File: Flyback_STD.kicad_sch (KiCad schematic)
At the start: 46 parts, among them P1 BATT+, P2 BATT-, P3 VBUS, P4 GND, Q1 5N20A, T1 TRF-6, U1 OB2106MP, U2 VPC2188B, U4 TL431

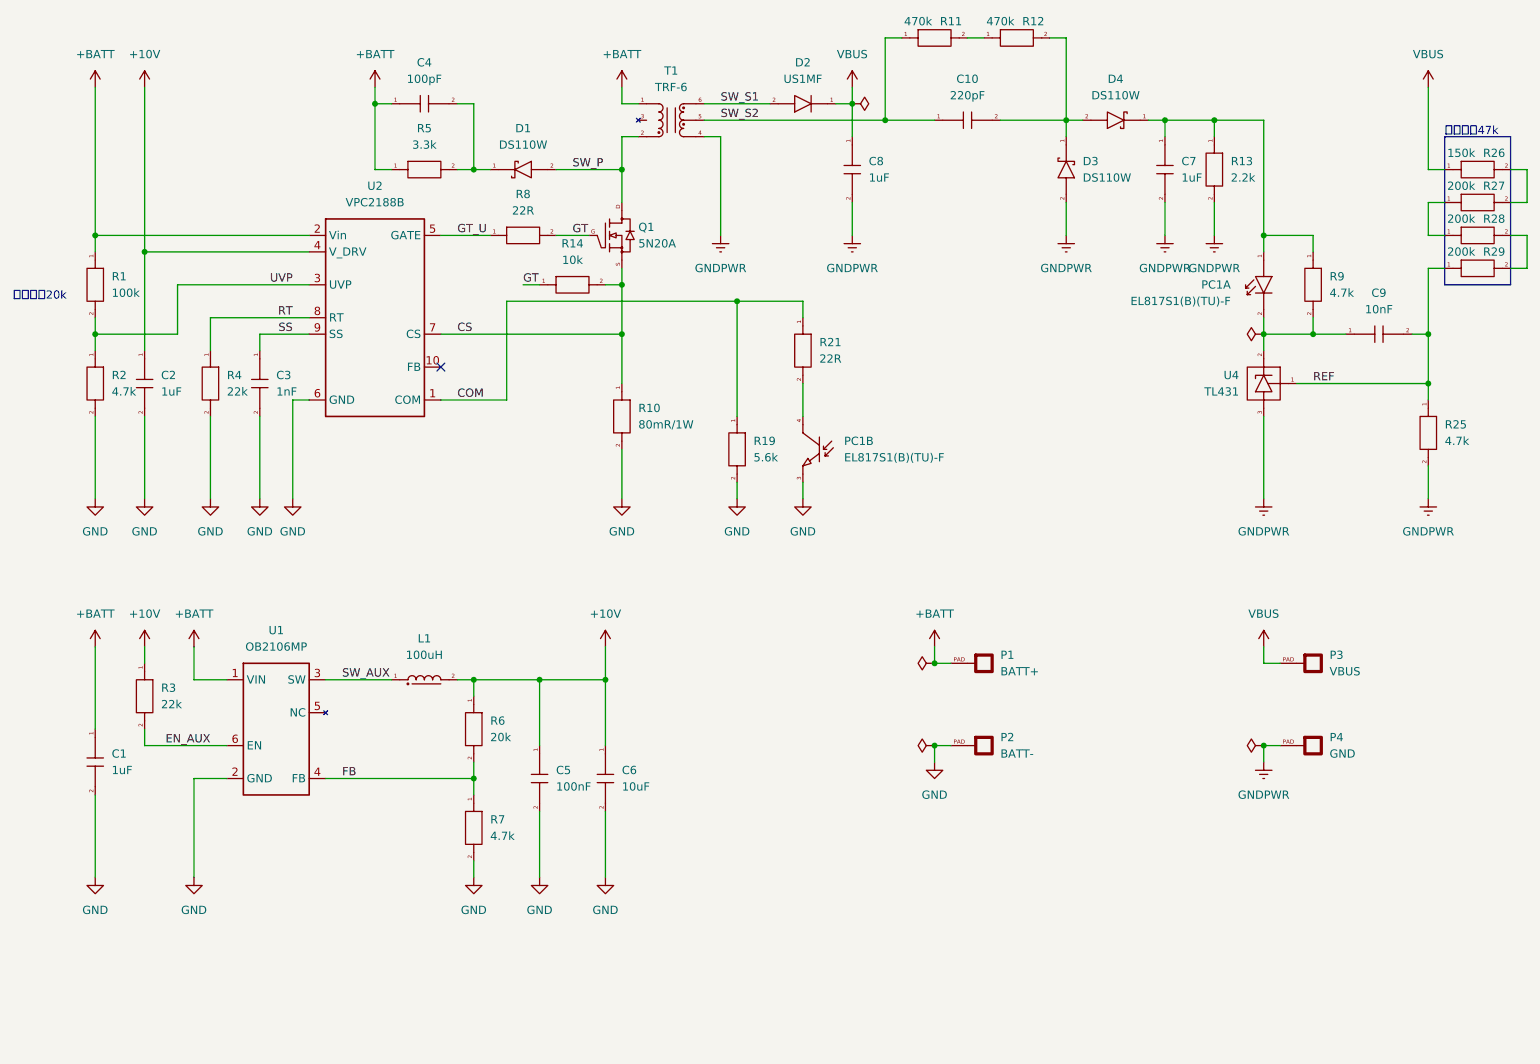
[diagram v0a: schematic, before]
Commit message: Daily update
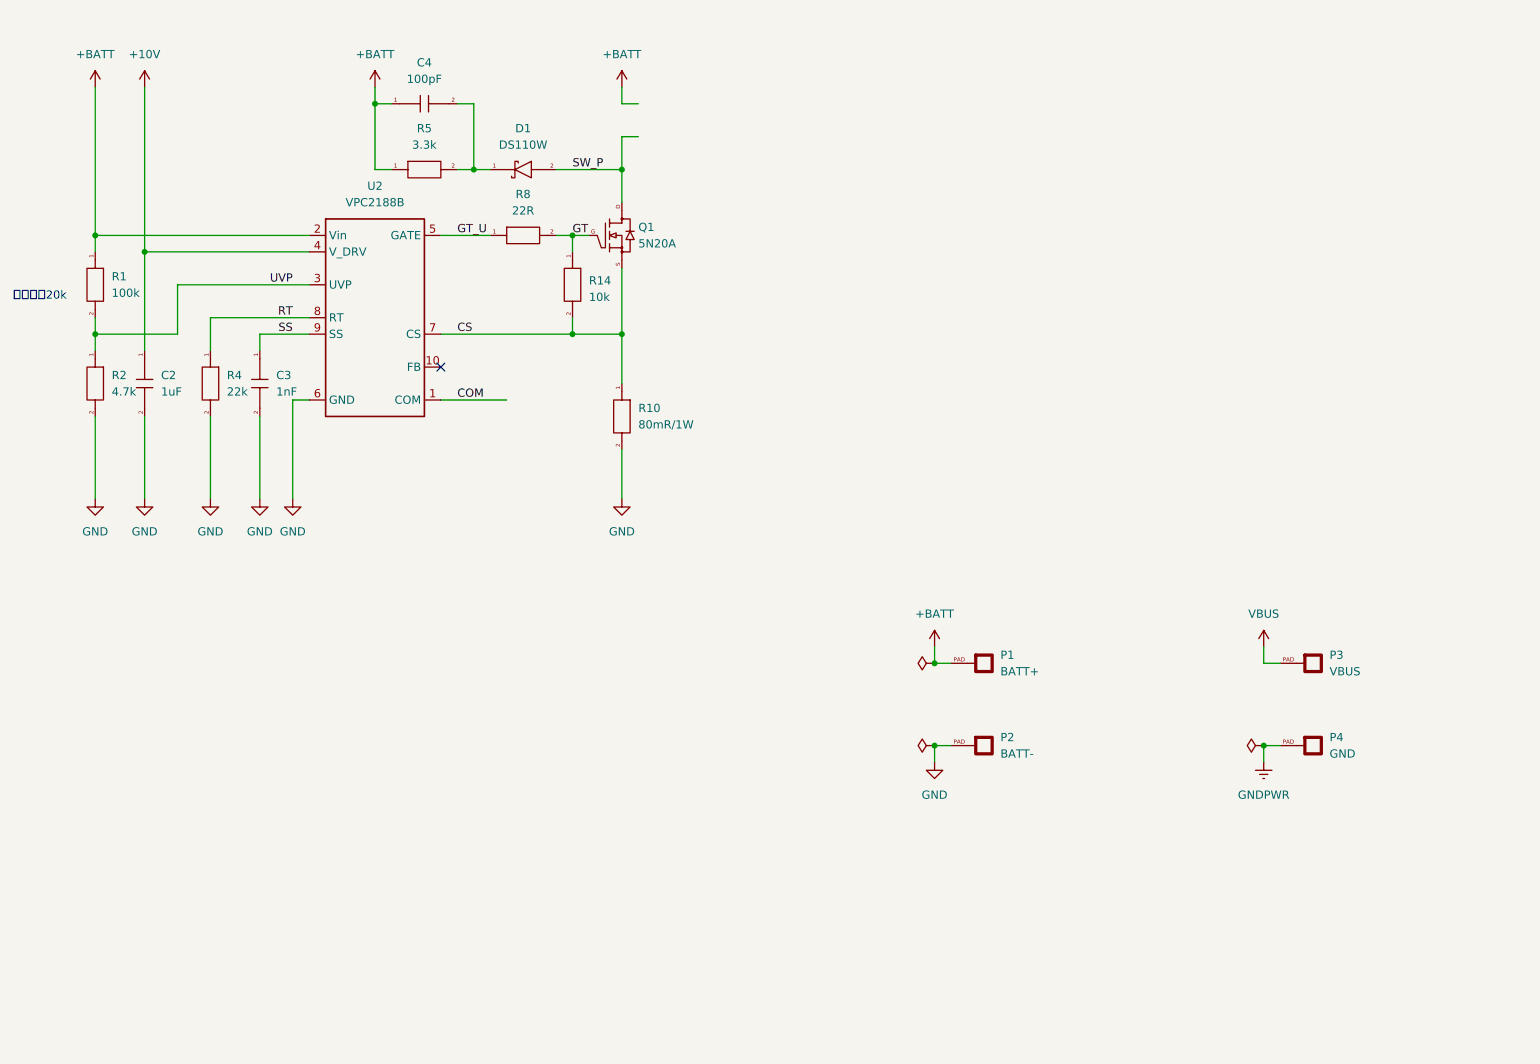
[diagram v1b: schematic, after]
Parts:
- removed C1: 1uF, 001_GN_RCL_SMD:C1206(3216M), symbol 001_Basic_PassiveComponents:101_Capacitor
- removed C10: 220pF, 001_GN_RCL_SMD:C1206(3216M), symbol 001_Basic_PassiveComponents:101_Capacitor
- removed C5: 100nF, 001_GN_RCL_SMD:C0603(1608M), symbol 001_Basic_PassiveComponents:101_Capacitor
- removed C6: 10uF, 001_GN_RCL_SMD:C0805(2012M), symbol 001_Basic_PassiveComponents:101_Capacitor
- removed C7: 1uF, 001_GN_RCL_SMD:C0805(2012M), symbol 001_Basic_PassiveComponents:101_Capacitor
- removed C8: 1uF, 001_GN_RCL_SMD:C2220(5650M), symbol 001_Basic_PassiveComponents:101_Capacitor
- removed C9: 10nF, 001_GN_RCL_SMD:C0603(1608M), symbol 001_Basic_PassiveComponents:101_Capacitor
- removed D2: US1MF, 002_GN_TWO-PIN_PLASTIC_SMD:SMA(DO-214AC), symbol 002_Basic_SingleSemiconductor:001_Diode
- removed D3, D4: DS110W, 002_GN_TWO-PIN_PLASTIC_SMD:SOD-123F, symbol 002_Basic_SingleSemiconductor:002_Diode_Schottky
- removed L1: 100uH, 008_GN_POWER-CHOKE_SMD:MC-0420, symbol 001_Basic_PassiveComponents:202_PowerChoke
- removed PC1: EL817S1(B)(TU)-F, MRLA:OC-4_6546, symbol MRLA:PC-4
- removed R11, R12: 470k, 001_GN_RCL_SMD:R0805(2012M), symbol 001_Basic_PassiveComponents:001_Resistor
- removed R13: 2.2k, 001_GN_RCL_SMD:R0603(1608M), symbol 001_Basic_PassiveComponents:001_Resistor
- removed R19: 5.6k, 001_GN_RCL_SMD:R0603(1608M), symbol 001_Basic_PassiveComponents:001_Resistor
- removed R21: 22R, 001_GN_RCL_SMD:R0603(1608M), symbol 001_Basic_PassiveComponents:001_Resistor
- removed R25, R7, R9: 4.7k, 001_GN_RCL_SMD:R0603(1608M), symbol 001_Basic_PassiveComponents:001_Resistor
- removed R26: 150k, 001_GN_RCL_SMD:R1206(3216M), symbol 001_Basic_PassiveComponents:001_Resistor
- removed R27, R28, R29: 200k, 001_GN_RCL_SMD:R1206(3216M), symbol 001_Basic_PassiveComponents:001_Resistor
- removed R3: 22k, 001_GN_RCL_SMD:R0603(1608M), symbol 001_Basic_PassiveComponents:001_Resistor
- removed R6: 20k, 001_GN_RCL_SMD:R0603(1608M), symbol 001_Basic_PassiveComponents:001_Resistor
- removed T1: TRF-6, MRLA:TRF-6_6P30S, symbol MRLA:TRF-6
- removed U1: OB2106MP, 003_GN_SMALL-SEMI_SMD:SOT-23-6, symbol 204_Power_SMPS-Convertor:OB2106MP
- removed U4: TL431, 003_GN_SMALL-SEMI_SMD:SOT-23, symbol 103_IntegratedCircuit_Reference:TL431
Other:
- note removed: "调试阶段47k"
- moved on the sheet: R14

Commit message: Nightly update
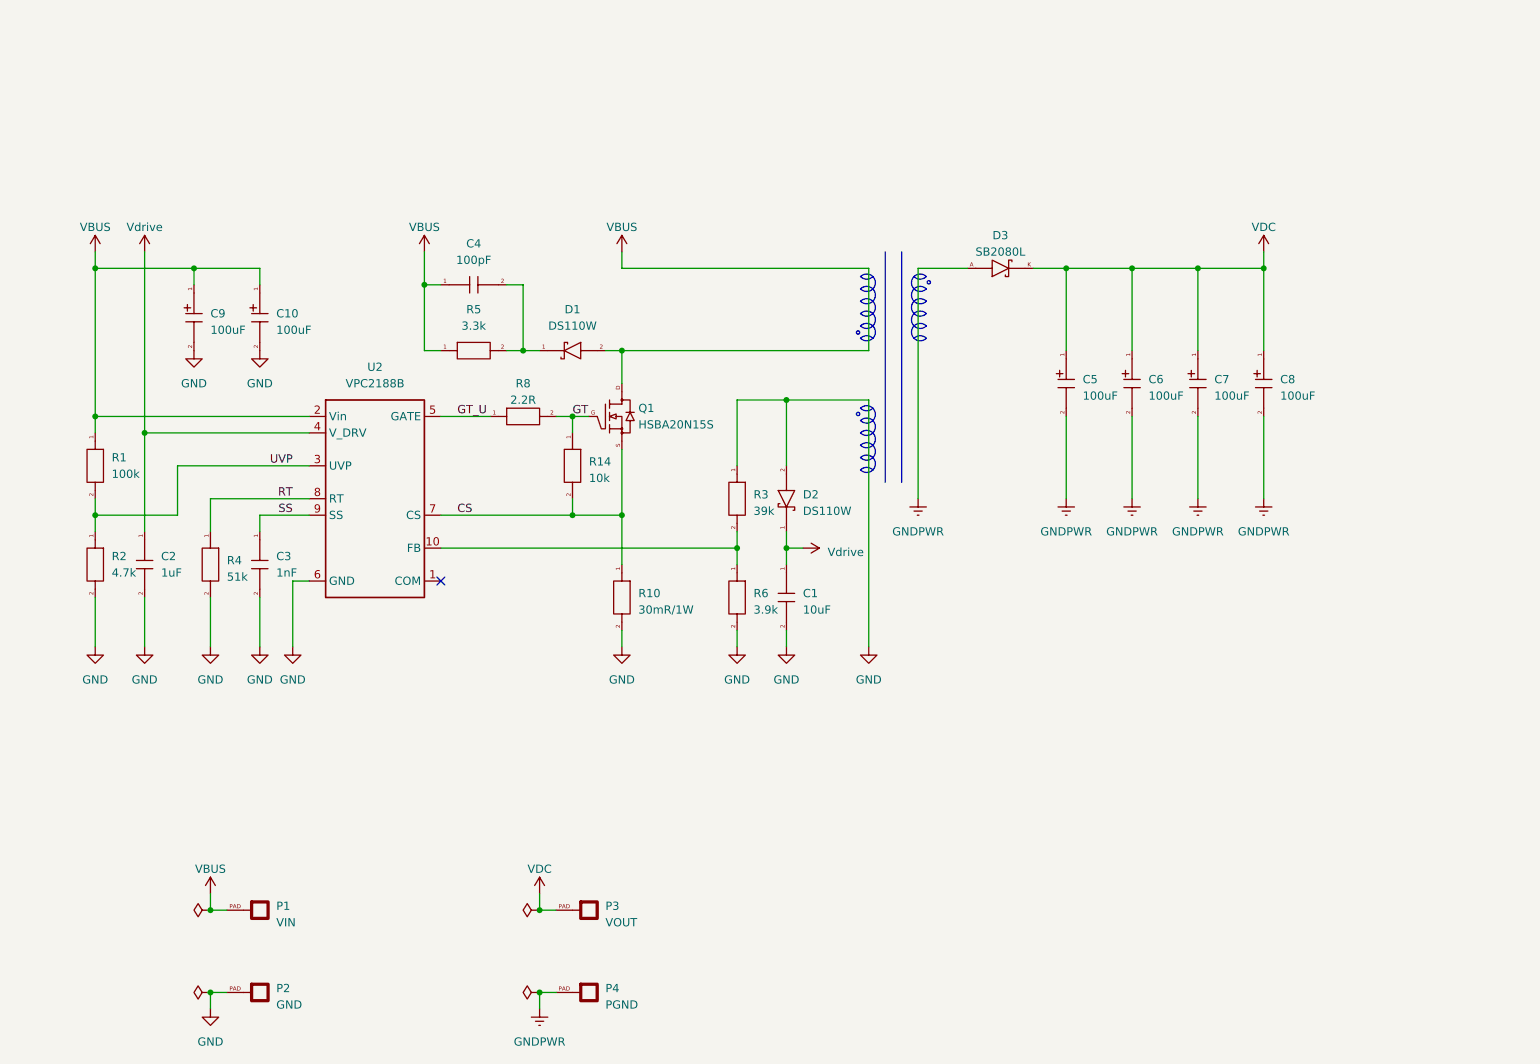
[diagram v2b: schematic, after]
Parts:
- added C1: 10uF, 001_GN_RCL_SMD:C0805(2012M), symbol 001_Basic_PassiveComponents:101_Capacitor
- added C10, C9: 100uF, 007_GN_POLAR-CAP_SMD:CL-1010, symbol 001_Basic_PassiveComponents:102_PolarCapacitor
- added C5, C6, C7, C8: 100uF, 007_GN_POLAR-CAP_SMD:CL-0608, symbol 001_Basic_PassiveComponents:102_PolarCapacitor
- added D2: DS110W, 002_GN_TWO-PIN_PLASTIC_SMD:SOD-123F, symbol 002_Basic_SingleSemiconductor:002_Diode_Schottky
- added D3: SB2080L, 102_SP_POWER_DIODE_SMD:TO-277A, symbol 201_Power_Diode:002_Diode_Schottky
- added R3: 39k, 001_GN_RCL_SMD:R0603(1608M), symbol 001_Basic_PassiveComponents:001_Resistor
- added R6: 3.9k, 001_GN_RCL_SMD:R0603(1608M), symbol 001_Basic_PassiveComponents:001_Resistor
- C4: footprint 001_GN_RCL_SMD:C0603(1608M) -> 001_GN_RCL_SMD:C0805(2012M)
- P1: value BATT+ -> VIN
- P2: value BATT- -> GND
- P3: value VBUS -> VOUT
- P4: value GND -> PGND
- Q1: value 5N20A -> HSBA20N15S; footprint 103_SP_POWER_TRANSISTOR_SMD:TO252-FET_6561 -> 103_SP_POWER_TRANSISTOR_SMD:SON-FET_6050; LCSC (none) -> C701044
- R10: value 80mR/1W -> 30mR/1W; LCSC (none) -> C2988649
- R4: value 22k -> 51k
- R8: value 22R -> 2.2R
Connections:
- net +BATT is gone; now on net VBUS: C4.1, P1.PAD, R1.1, R5.1, U2.2 (Vin)
- net SW_P is gone; now on net VBUS: D1.2 (Anode), Q1.D (Drain)
- net GND: now also C1.2, C10.2, C9.2, D2.2 (Anode), R3.1, R6.2
- net GNDPWR: now also C5.2, C6.2, C7.2, C8.2, D3.A (Anode)
- net VBUS: now also C10.1, C9.1; no longer P3.PAD
- net at U2.10 (FB): now also R3.2, R6.1
- net +10V renamed Vdrive
- net Vdrive: now also C1.1, D2.1 (Cathode)
- net COM: no longer names the net of U2.1 (COM)
- new net VDC: C5.1, C6.1, C7.1, C8.1, D3.K (Cathode), P3.PAD
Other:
- note removed: "调试阶段20k"
- moved on the sheet: C2, C3, C4, D1, P1, P2, P3, P4, Q1, R1, R10, R14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
